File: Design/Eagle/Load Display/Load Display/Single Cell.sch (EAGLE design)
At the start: 12 parts

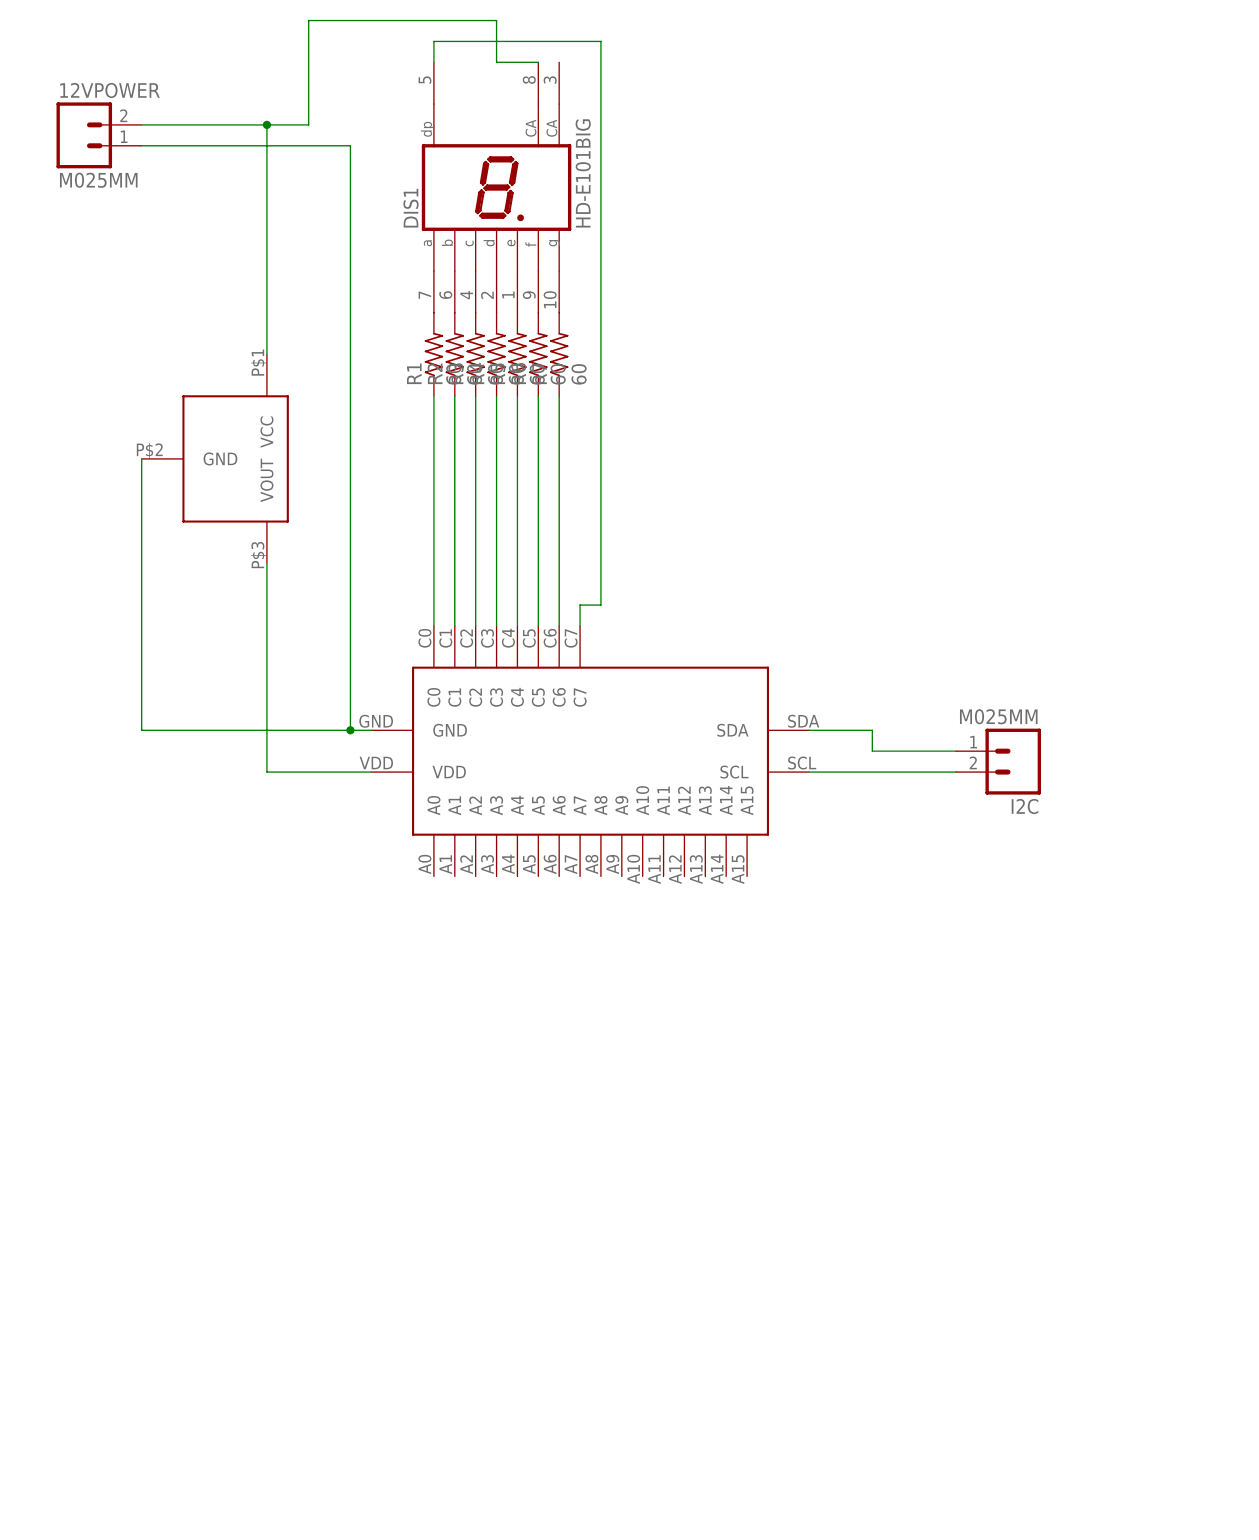
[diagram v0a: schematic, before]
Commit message: Merge remote-tracking branch 'remotes/origin/Panic_Mode_Ben' into HEAD
Conflicts:
	Python/Master.py
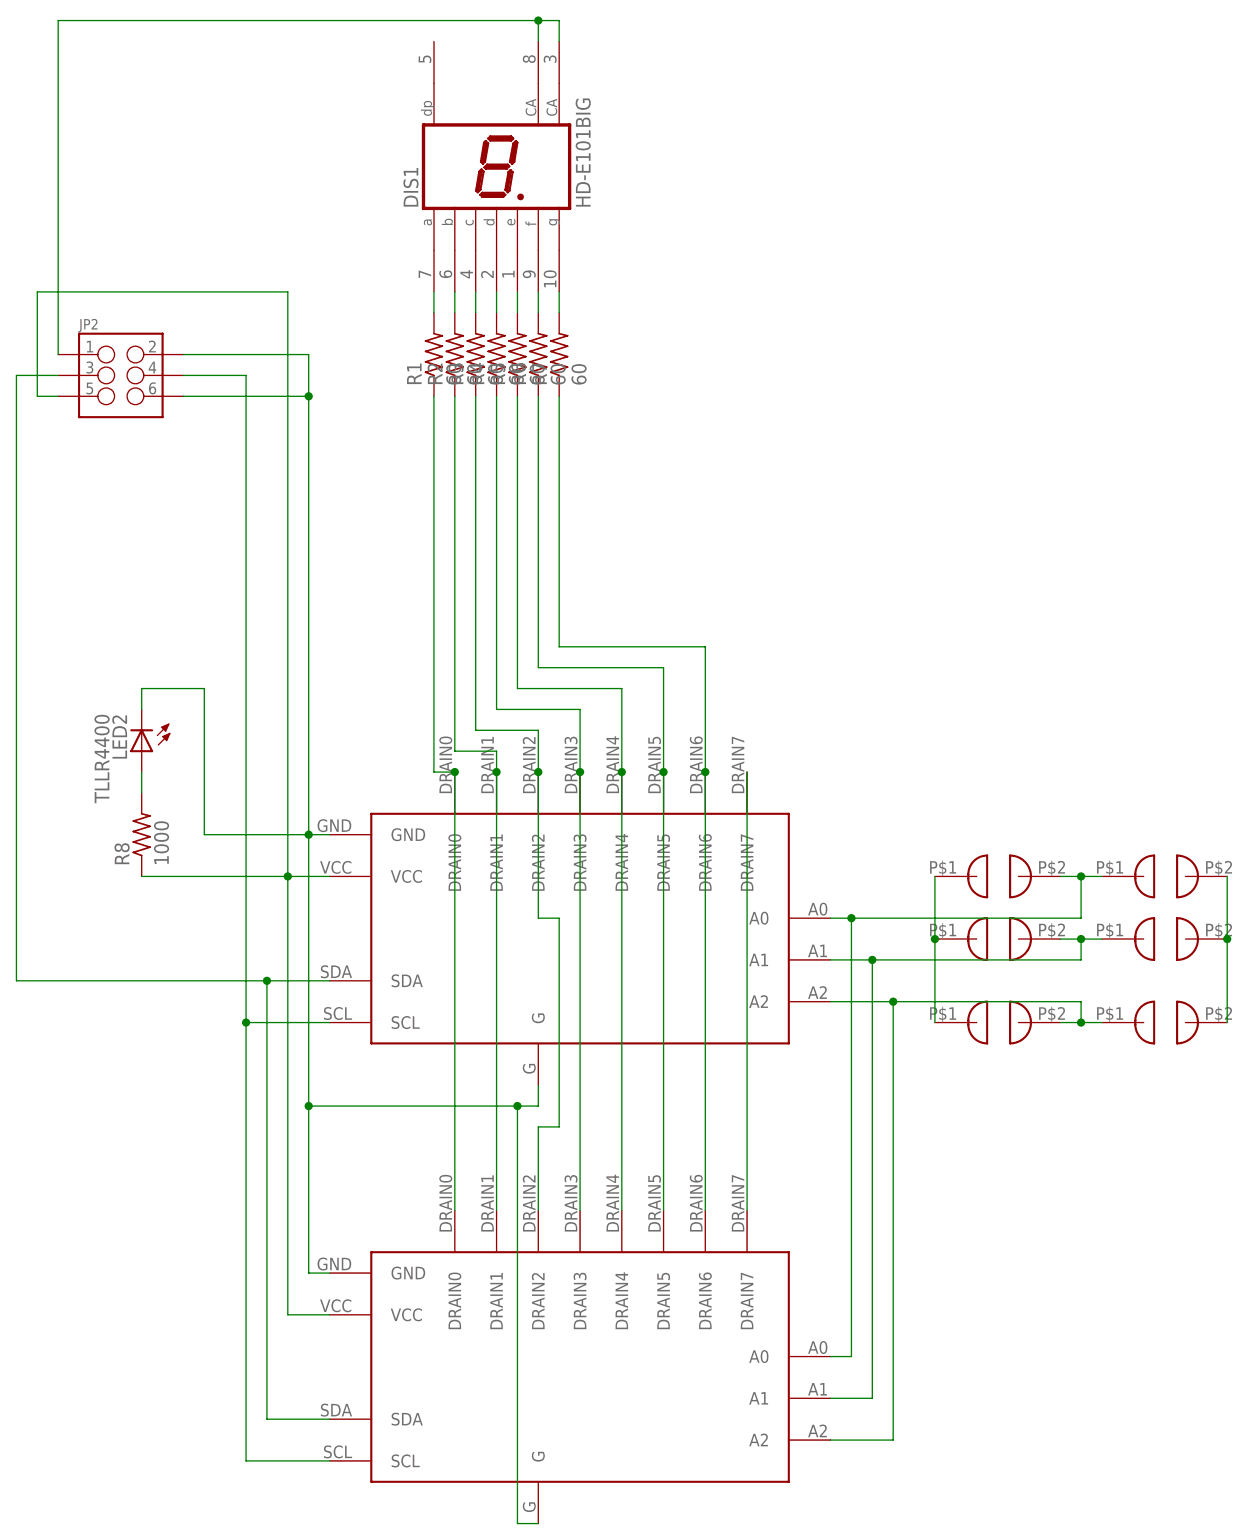
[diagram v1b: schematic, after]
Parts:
- removed 12VPOWER, I2C: M025MM, Ben-SF-Con:M025MM
- added JP2: (no value), Ben-SF-Con:M03X2SHROUD
- added LED2: TLLR4400, led:TLLR4400
- added R8: 1000, Ben-rcl:R-US_0207/15
- added U$2: (no value), Parts:LED_DRIVERBOARDADAFRUIT
- added U$4, U$5, U$6, U$7: SOLDER_JUMPER, Parts:SOLDER_JUMPER
- added U$8: (no value), Parts:LED_DRIVERBOARD
- DIS1: device Parts:HD-E101BIG -> Parts:HD-E101BACKWARDS
- R1, R2, R3, R4, R5: device Ben-rcl:R-US_0207/10 -> Ben-rcl:R-US_0207/15
- U$1: value 5VREG -> SOLDER_JUMPER; device Parts:5VREG -> Parts:SOLDER_JUMPER
- U$3: value HT16K33BRD -> SOLDER_JUMPER; device Parts:HT16K33BRD -> Parts:SOLDER_JUMPER
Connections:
- removed net N$19: U$1.VOUT, U$3.VDD
- removed net N$20: 12VPOWER.2, DIS1.CA@1, U$1.VCC
- new net GND: JP2.2, JP2.6, LED2.C, U$1.P$3, U$2.G, U$2.GND, U$4.P$3, U$6.P$3, U$8.G, U$8.GND
- new net N$29: U$1.P$4, U$2.A0, U$3.P$3, U$8.A0
- new net SDA: JP2.3, U$2.SDA, U$8.SDA
- new net SSCL: JP2.4, U$2.SCL, U$8.SCL
- new net VCC12: DIS1.CA, DIS1.CA@1, JP2.1
- new net VCC5: JP2.5, R8.1, U$2.VCC, U$3.P$4, U$5.P$4, U$7.P$4, U$8.VCC
- net N$10: now also U$2.DRAIN2, U$8.DRAIN2; no longer U$3.C2
- net N$11: now also U$2.DRAIN3, U$8.DRAIN3; no longer U$3.C3
- net N$12: now also U$2.DRAIN4, U$8.DRAIN4; no longer U$3.C4
- net N$13: now also U$2.DRAIN5, U$8.DRAIN5; no longer U$3.C5
- net N$14: now also U$2.DRAIN6, U$8.DRAIN6; no longer U$3.C6
- net N$15: now also U$2.A1, U$4.P$4, U$5.P$3, U$8.A1; no longer I2C.1, U$3.SDA
- net N$16: now also U$2.A2, U$6.P$4, U$7.P$3, U$8.A2; no longer I2C.2, U$3.SCL
- net N$17: now also U$2.DRAIN7, U$8.DRAIN7; no longer 12VPOWER.1, U$1.GND, U$3.GND
- net N$18: now also LED2.A, R8.2; no longer DIS1.DP, U$3.C7
- net N$8: now also U$2.DRAIN0, U$8.DRAIN0; no longer U$3.C0
- net N$9: now also U$2.DRAIN1, U$8.DRAIN1; no longer U$3.C1
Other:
- moved on the sheet: DIS1
